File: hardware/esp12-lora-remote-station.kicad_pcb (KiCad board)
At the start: 2 copper layers, 95 x 95 mm, 104 parts, among them J1 LM75_HEADER, J10 ROT_ENC_HEADER, J11 I2C_HEADER,2.54, J12 5V_header, J13 5V_header, J2 I2C_HEADER,2.54, J3 P0_HEADER, J4 P1_HEADER, J5 I2C_HEADER,2.54, J6 I2C_HEADER, J7 GSM_TX_HEADER, J8 I2C_HEADER,2.54, J9 I2C_HEADER,2.54, Q1 SS9013_J3, Q2 SS9013_J3, SW1 FLASH_BUTTON, SW2 SW_RESET,2_leg,SMD, SW3 USER_BUTTON1, SW4 USER_BUTTON2, SW5 USER_BUTTON1, SW6 EC11_VERTICAL, U1 LM75, U2 SHT20, U3 PCF8575C, U4 ESP12, U5 AMS1117-3.3, U6 USB_Micro, U7 CP2102, U8 SSD1306-OLED-I2C, U9 74AHCT1G125

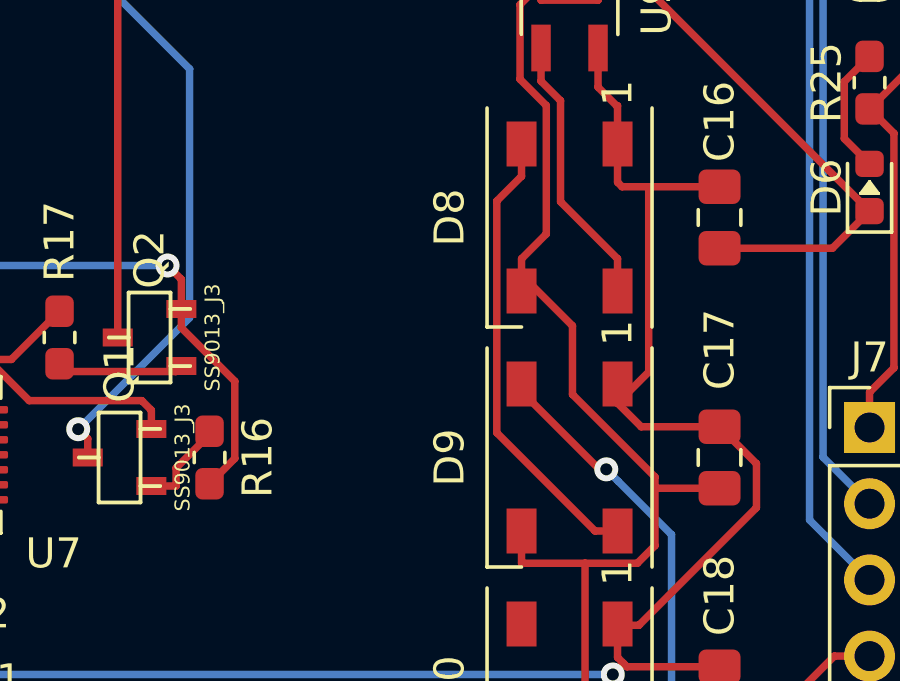
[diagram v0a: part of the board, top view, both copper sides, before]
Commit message: update DRC ok,
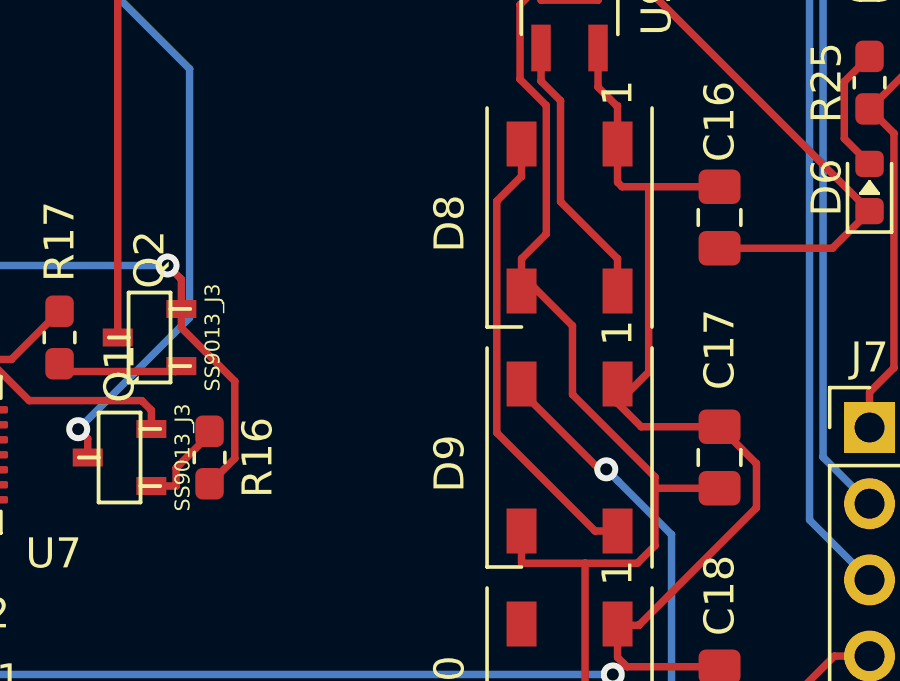
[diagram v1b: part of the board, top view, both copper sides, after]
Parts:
- D10, D8, D9: footprint LED_SMD:LED_WS2812B_PLCC4_5.0x5.0mm_P3.2mm -> footprint-lib:LED_WS2812B_5050_white
